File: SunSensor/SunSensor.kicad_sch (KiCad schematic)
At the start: 19 parts, among them U1 AD7291BCPZ, U2 FEATHER_M0_BASIC_PROTO

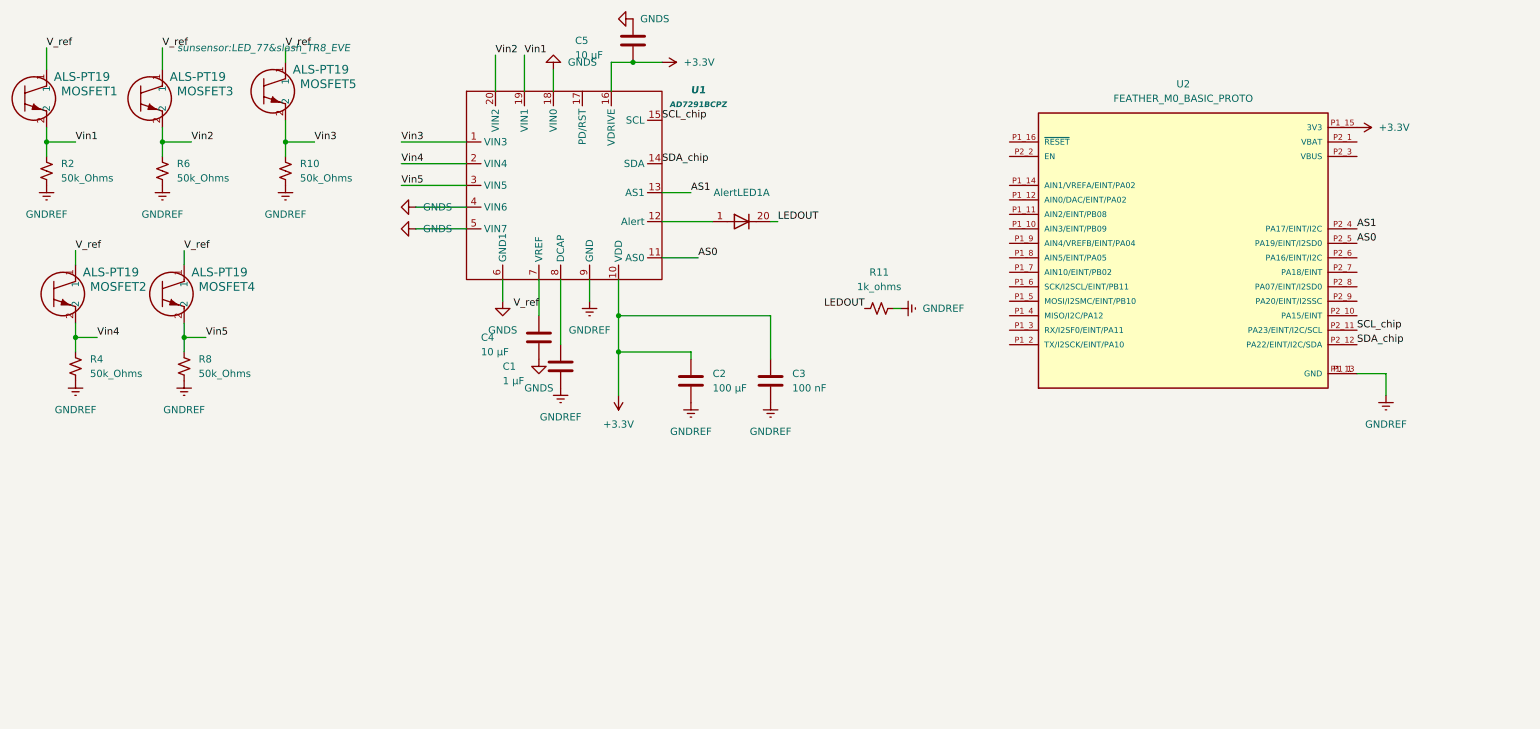
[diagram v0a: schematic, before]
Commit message: Finish Routing
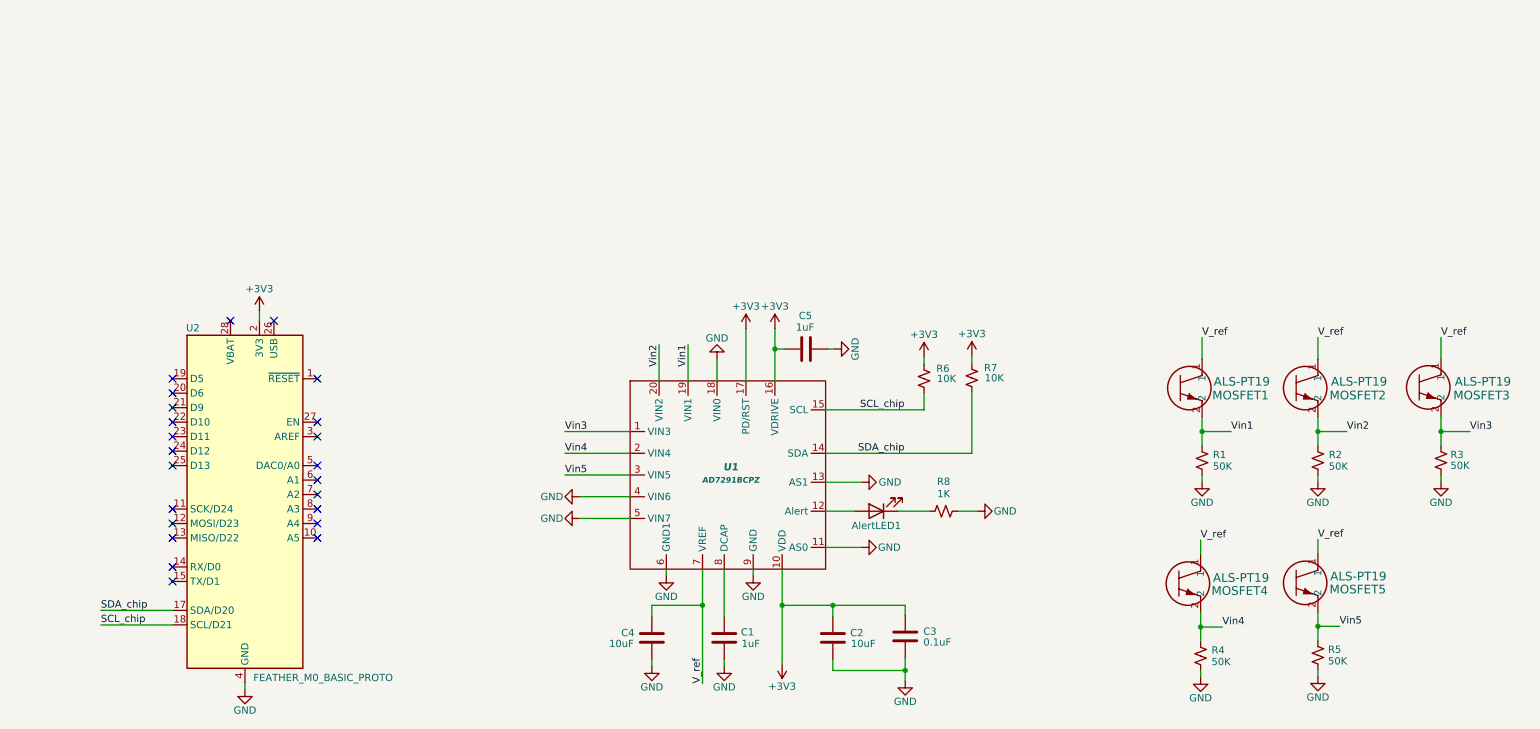
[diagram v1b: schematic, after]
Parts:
- added R6, R7: 10K, Resistor_SMD:R_0603_1608Metric, symbol Device:R_Small_US
- AlertLED1: footprint sunsensor:LED_77&slash_TR8_EVE -> LED_SMD:LED_0603_1608Metric; symbol LED:HDSP-4836 -> Device:LED
- C1: value 1 µF -> 1uF; footprint sunsensor:CAPC1005X60N -> Capacitor_SMD:C_0603_1608Metric
- C2: value 100 µF -> 10uF; footprint sunsensor:CAPC3216X190N -> Capacitor_SMD:C_0603_1608Metric
- C3: value 100 nF -> 0.1uF; footprint sunsensor:CAPC1005X55N -> Capacitor_SMD:C_0603_1608Metric
- C4: value 10 µF -> 10uF; footprint sunsensor:CAPC1005X71N -> Capacitor_SMD:C_0603_1608Metric
- C5: value 10 µF -> 1uF; footprint sunsensor:CAPC1005X71N -> Capacitor_SMD:C_0603_1608Metric
- MOSFET1: symbol 4xxx:ALS-PT19-315C_L177_TR8 -> SunSensor:ALS-PT19
- MOSFET2: renamed from MOSFET3; symbol 4xxx:ALS-PT19-315C_L177_TR8 -> SunSensor:ALS-PT19
- MOSFET3: renamed from MOSFET5; symbol 4xxx:ALS-PT19-315C_L177_TR8 -> SunSensor:ALS-PT19
- MOSFET4: renamed from MOSFET2; symbol 4xxx:ALS-PT19-315C_L177_TR8 -> SunSensor:ALS-PT19
- MOSFET5: renamed from MOSFET4; symbol 4xxx:ALS-PT19-315C_L177_TR8 -> SunSensor:ALS-PT19
- R1: renamed from R2; value 50k_Ohms -> 50K; footprint sunsensor:RESC3116X65N -> Resistor_SMD:R_0603_1608Metric; symbol Device:50k_Ohms -> Device:R_Small_US
- R2: renamed from R6; value 50k_Ohms -> 50K; footprint sunsensor:RESC3116X65N -> Resistor_SMD:R_0603_1608Metric; symbol Device:50k_Ohms -> Device:R_Small_US
- R3: renamed from R10; value 50k_Ohms -> 50K; footprint sunsensor:RESC3116X65N -> Resistor_SMD:R_0603_1608Metric; symbol Device:50k_Ohms -> Device:R_Small_US
- R4: value 50k_Ohms -> 50K; footprint sunsensor:RESC3116X65N -> Resistor_SMD:R_0603_1608Metric; symbol Device:50k_Ohms -> Device:R_Small_US
- R5: renamed from R8; value 50k_Ohms -> 50K; footprint sunsensor:RESC3116X65N -> Resistor_SMD:R_0603_1608Metric; symbol Device:50k_Ohms -> Device:R_Small_US
- R8: renamed from R11; value 1k_ohms -> 1K; footprint sunsensor:RESC3216X75N -> Resistor_SMD:R_0603_1608Metric; symbol Device:50k_Ohms -> Device:R_Small_US
- U1: footprint sunsensor:QFN50P400X400X100-21N -> Package_DFN_QFN:QFN-20-1EP_4x4mm_P0.5mm_EP2.6x2.6mm; symbol Analog_ADC:AD7291BCPZ -> SunSensor:AD7291BCPZ
- U2: footprint MODULE_FEATHER_M0_BASIC_PROTO -> Module:Adafruit_Feather; symbol sunsensor:FEATHER_M0_BASIC_PROTO -> MCU_Module:Adafruit_Feather_M0_Basic_Proto
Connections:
- net GNDS is gone; now on net GND: C4.2, C5.1, U1.18 (VIN0), U1.4 (VIN6), U1.5 (VIN7), U1.6 (GND1)
- net +3V3: now also U1.17 (PD/RST), U2.2 (3V3), R6.2, R7.2; no longer U2.P1_15 (3V3)
- net SCL_chip: now also U2.18 (SCL/D21), R6.1; no longer U2.P2_11 (PA23/EINT/I2C/SCL)
- net SDA_chip: now also U2.17 (SDA/D20), R7.1; no longer U2.P2_12 (PA22/EINT/I2C/SDA)
- net at U1.12 (Alert): now also AlertLED1.2 (A); no longer AlertLED1.1 (A)
- net AS0 renamed GND
- net GND: now also C1.2, C2.2, C3.2, R1.2, R2.2, R3.2, R4.2, R5.2, R8.2, U1.13 (AS1), U1.21 (GND), U1.9 (GND), U2.16 (GND), U2.4 (GND); no longer U2.P2_5 (PA19/EINT/I2SD0)
- removed net AS1: U1.13 (AS1), U2.P2_4 (PA17/EINT/I2C)
- removed net GNDREF: C1.2, C2.2, C3.2, R1.2, R2.2, R3.2, R4.2, R5.2, R8.2, U1.9 (GND), U2.P1_1 (GND), U2.P1_13 (GND)
- net LEDOUT: no longer names the net of R8.1
- net LEDOUT: now also AlertLED1.1 (K); no longer AlertLED1.20 (K)
- no-connect marks 0 -> 23
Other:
- moved on the sheet: AlertLED1, C1, C2, C3, C5, MOSFET1, MOSFET2, MOSFET3, MOSFET4, MOSFET5, R1, R2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
